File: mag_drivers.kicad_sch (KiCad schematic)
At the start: 29 parts, among them J10 Conn_01x02_Pin, J11 Conn_01x02_Pin, J9 Conn_01x02_Pin, U11 STSPIN250, U2 STSPIN250, U24 AP22652, U8 STSPIN250

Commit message: started layout
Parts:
- C69, C79, C82: footprint (none) -> Capacitor_SMD:C_0201_0603Metric
- J10, J11, J9: footprint (none) -> Connector_JST:JST_SH_BM02B-SRSS-TB_1x02-1MP_P1.00mm_Vertical
- R14, R15, R23, R24, R60, R61, R62, R63, R64: footprint (none) -> Resistor_SMD:R_0402_1005Metric
- R65: footprint Resistor_SMD:R_0603_1608Metric -> Resistor_SMD:R_0402_1005Metric
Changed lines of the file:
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@@
 			)
 		)
-		(property "Footprint" ""
+		(property "Footprint" "Resistor_SMD:R_0402_1005Metric"
 			(at 245.11 135.89 0)
 			(effects
@@
 			)
 		)
-		(property "Footprint" ""
+		(property "Footprint" "Resistor_SMD:R_0402_1005Metric"
 			(at 242.57 64.77 0)
 			(effects
@@
 			)
 		)
-		(property "Footprint" ""
+		(property "Footprint" "Resistor_SMD:R_0402_1005Metric"
 			(at 35.56 46.99 0)
 			(effects
@@
 			)
 		)
-		(property "Footprint" ""
+		(property "Footprint" "Resistor_SMD:R_0402_1005Metric"
 			(at 100.33 63.5 0)
 			(effects
@@
 			)
 		)
-		(property "Footprint" ""
+		(property "Footprint" "Connector_JST:JST_SH_BM02B-SRSS-TB_1x02-1MP_P1.00mm_Vertical"
 			(at 262.89 127 0)
 			(effects
@@
 			)
 		)
-		(property "Footprint" "Resistor_SMD:R_0603_1608Metric"
+		(property "Footprint" "Resistor_SMD:R_0402_1005Metric"
 			(at 55.88 133.35 0)
 			(effects
@@
 			)
 		)
-		(property "Footprint" ""
+		(property "Footprint" "Resistor_SMD:R_0402_1005Metric"
 			(at 180.34 123.19 0)
 			(effects
@@
 			)
 		)
-		(property "Footprint" ""
+		(property "Footprint" "Capacitor_SMD:C_0201_0603Metric"
 			(at 170.18 52.07 0)
 			(effects
@@
 			)
 		)
-		(property "Footprint" ""
+		(property "Footprint" "Capacitor_SMD:C_0201_0603Metric"
 			(at 27.94 50.8 0)
 			(effects
@@
 			)
 		)
-		(property "Footprint" ""
+		(property "Footprint" "Resistor_SMD:R_0402_1005Metric"
 			(at 35.56 50.8 0)
 			(effects
@@
 			)
 		)
-		(property "Footprint" ""
+		(property "Footprint" "Resistor_SMD:R_0402_1005Metric"
 			(at 177.8 52.07 0)
 			(effects
@@
 			)
 		)
-		(property "Footprint" ""
+		(property "Footprint" "Connector_JST:JST_SH_BM02B-SRSS-TB_1x02-1MP_P1.00mm_Vertical"
 			(at 260.35 55.88 0)
 			(effects
@@
 			)
 		)
-		(property "Footprint" ""
+		(property "Footprint" "Resistor_SMD:R_0402_1005Metric"
 			(at 180.34 119.38 0)
 			(effects
@@
 			)
 		)
-		(property "Footprint" ""
+		(property "Footprint" "Connector_JST:JST_SH_BM02B-SRSS-TB_1x02-1MP_P1.00mm_Vertical"
 			(at 118.11 54.61 0)
 			(effects
@@
 			)
 		)
-		(property "Footprint" ""
+		(property "Footprint" "Resistor_SMD:R_0402_1005Metric"
 			(at 177.8 48.26 0)
 			(effects
@@
 			)
 		)
-		(property "Footprint" ""
+		(property "Footprint" "Capacitor_SMD:C_0201_0603Metric"
 			(at 172.72 123.19 0)
 			(effects

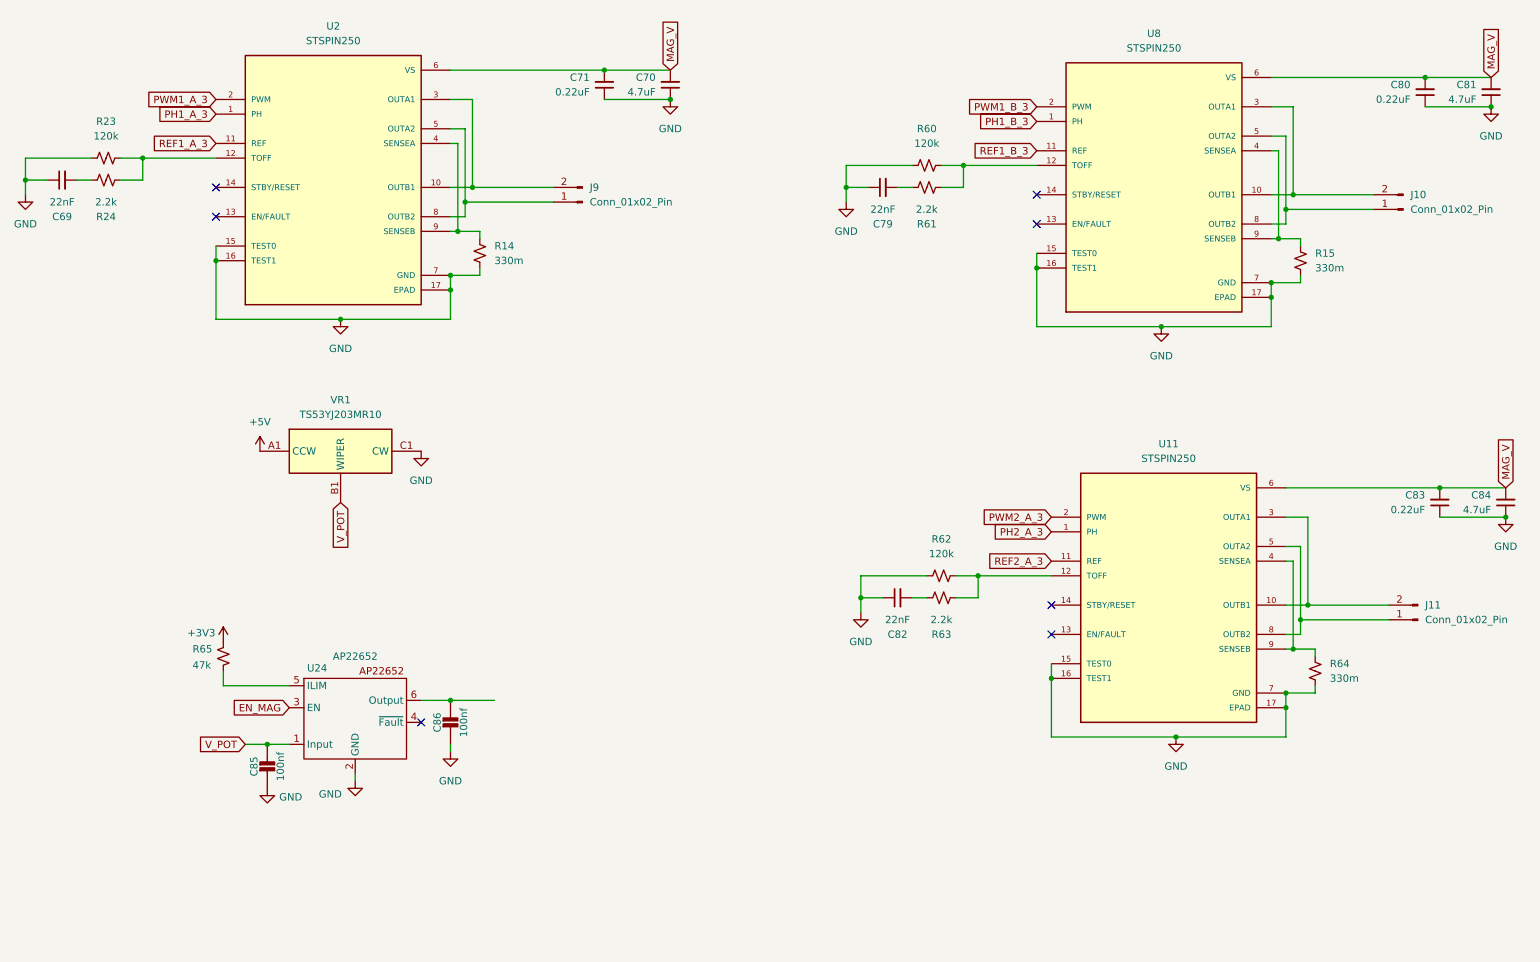
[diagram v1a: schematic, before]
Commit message: finished layout of v0.2!
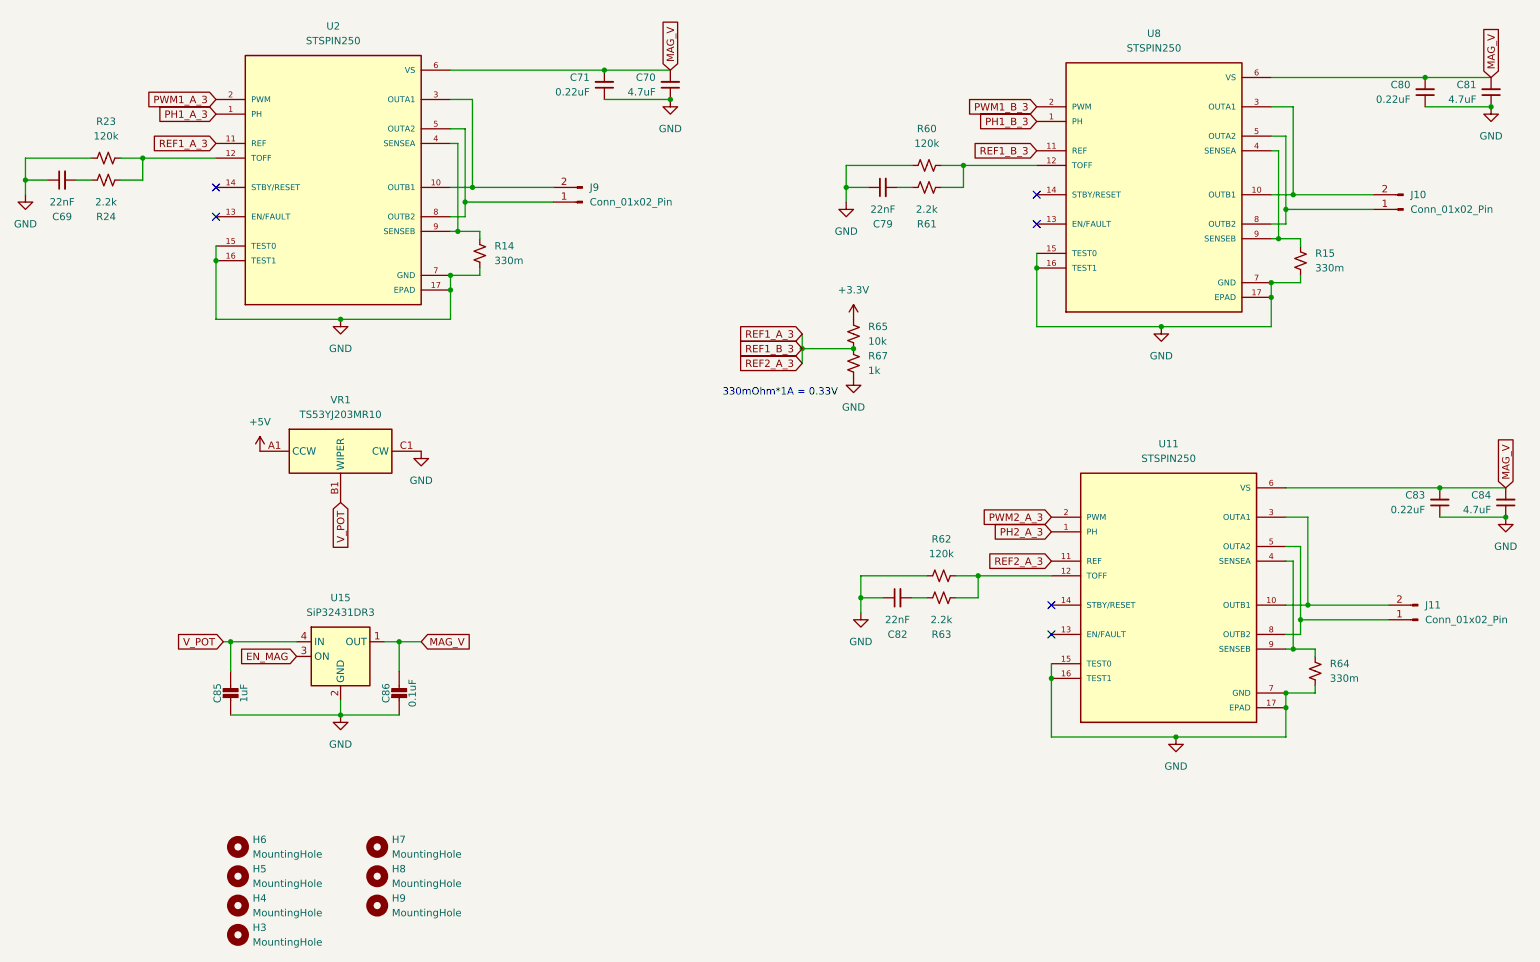
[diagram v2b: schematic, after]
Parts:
- removed U24: AP22652, SOT26:SOT26, symbol Power_Management:AP22652
- added H3, H4, H5, H6, H7, H8, H9: MountingHole, MountingHole:MountingHole_2.5mm_Pad, symbol Mechanical:MountingHole
- added R67: 1k, Resistor_SMD:R_0402_1005Metric, symbol Device:R_Small_US
- added U15: SiP32431DR3, Package_TO_SOT_SMD:SOT-363_SC-70-6, symbol Power_Management:SiP32431DR3
- C85: value 100nf -> 1uF
- C86: value 100nf -> 0.1uF
- R65: value 47k -> 10k; DPN RMCF0603FT47K0CT-ND -> (none); DST Digi-Key -> (none); MFR Stackpole Electronics Inc -> (none); MPN RMCF0603FT47K0 -> (none)
- U11, U2, U8: footprint STSPIN250:QFN50P300X300X100-17N -> footprints:QFN50P300X300X100-17N
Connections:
- net +3V3 is gone; now on net REF1_A_3: R65.1
- net REF1_B_3 is gone; now on net REF1_A_3: U8.11 (REF)
- net REF2_A_3 is gone; now on net REF1_A_3: U11.11 (REF)
- net EN_MAG: now also U15.3 (ON)
- net GND: now also R67.1, U15.2 (GND), U15.5 (GND)
- net MAG_V: now also C86.1, U15.1 (OUT)
- net REF1_A_3: now also R67.2
- net V_POT: now also U15.4 (IN)
- net +3.3V: now reaches R65.2
- no-connect marks 7 -> 6
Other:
- note added: "330mOhm*1A = 0.33V"
- moved on the sheet: C85
